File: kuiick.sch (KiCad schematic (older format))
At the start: 22 parts, among them J1 10118193-0001LF, J2 I2C_STANDARDQWIIC, J3 Conn_01x07, J4 Conn_01x07, SW1 SW_SPST, SW2 SW_SPST, U1 MK32L2B_QFN32, U2 W25Q32JVSS

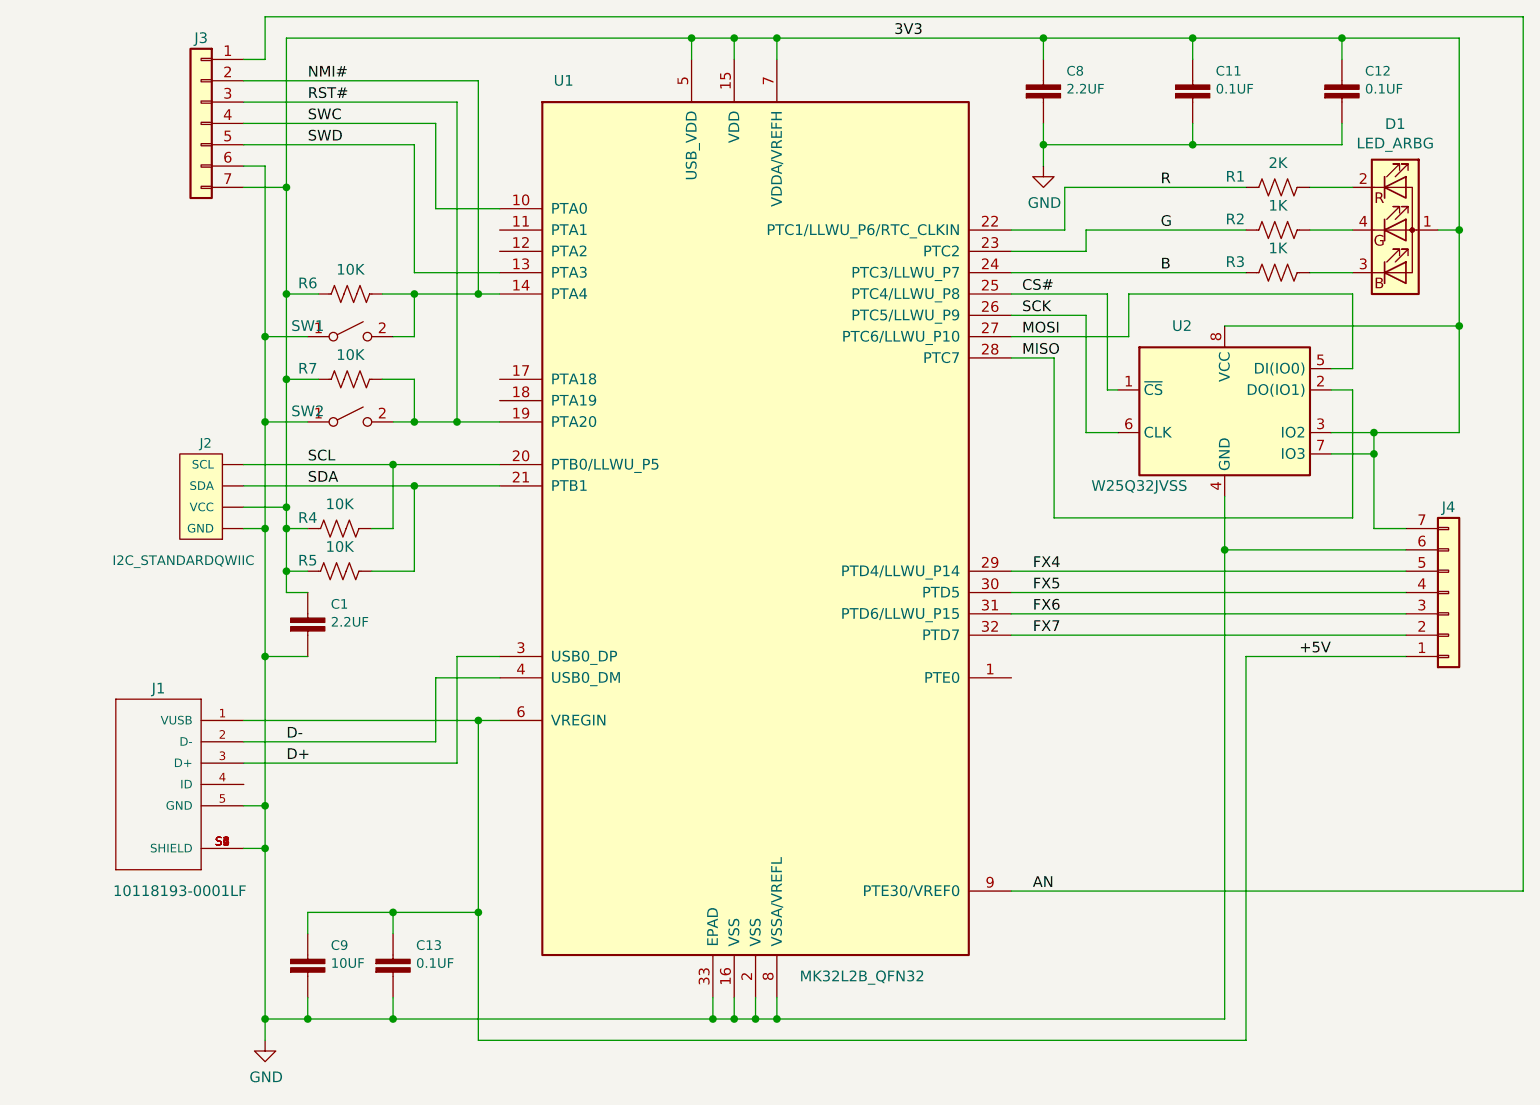
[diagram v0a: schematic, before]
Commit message: fully routed dip 16
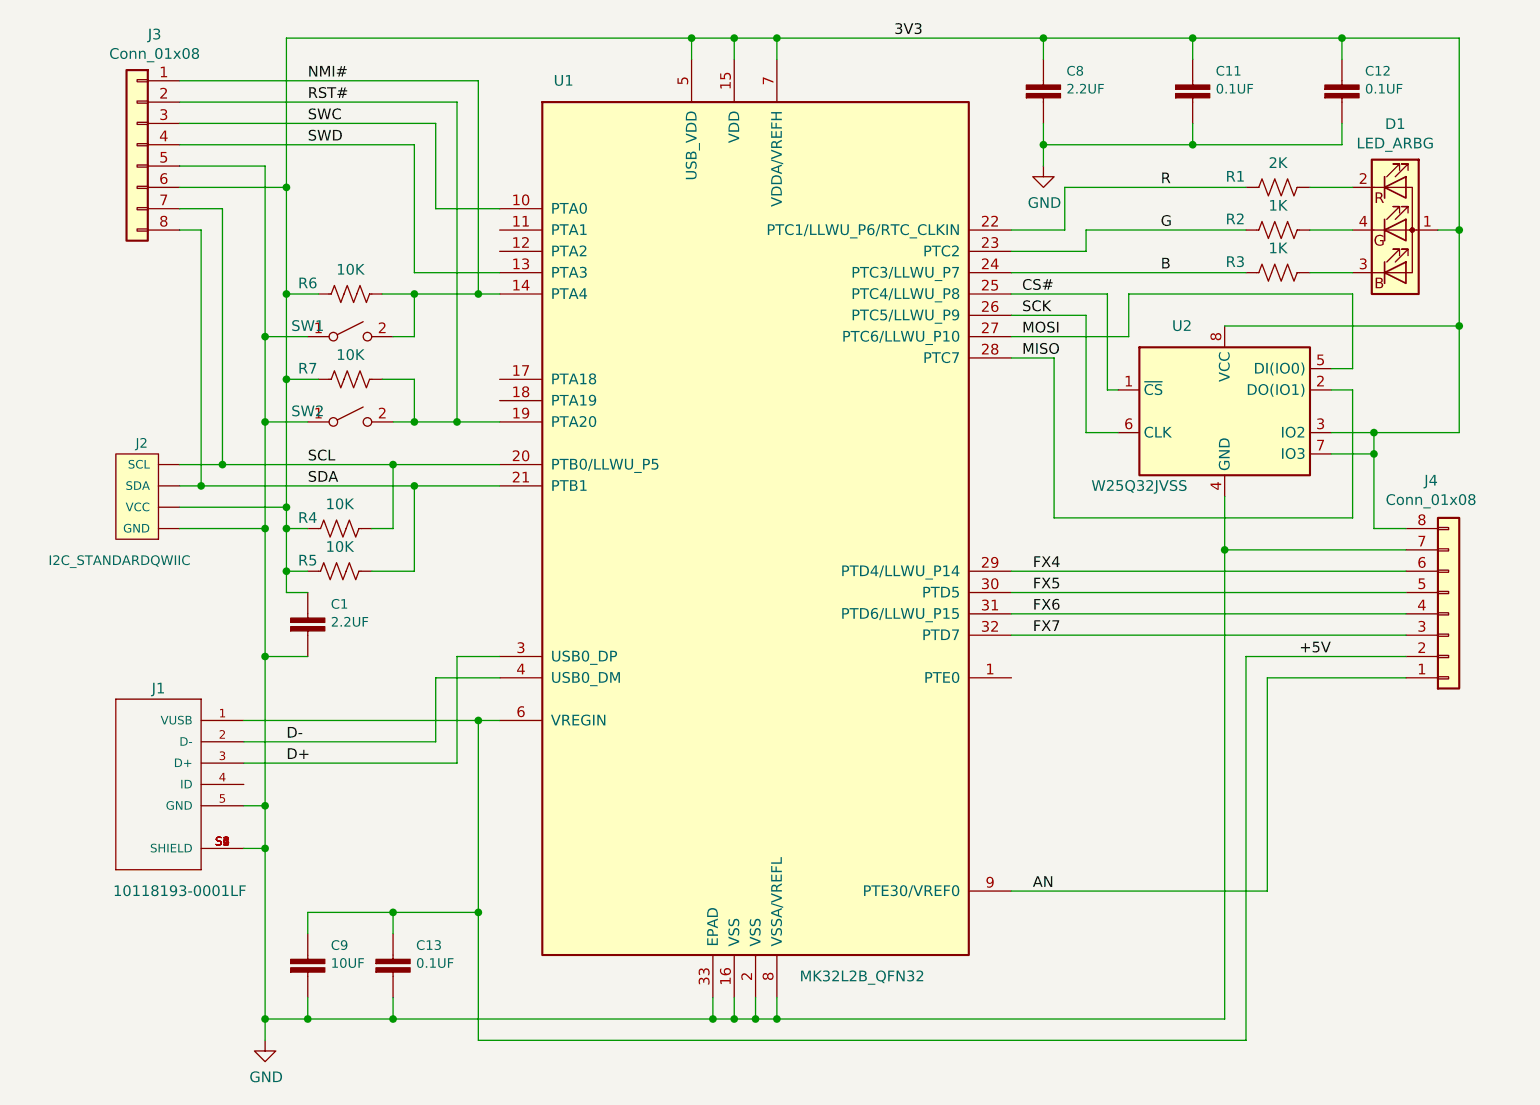
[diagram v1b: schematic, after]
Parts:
- removed J3, J4: Conn_01x07, footprint:PinHeader_1x07_P100mil_Vertical, symbol Connector_Generic:Conn_01x07
- added J3, J4: Conn_01x08, footprint:PinHeader_1x08_P100mil_Vertical, symbol Connector_Generic:Conn_01x08
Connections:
- net +5V: now also J4.2 (Pin_2)
- net 3V3: now also J3.6 (Pin_6), J4.8 (Pin_8)
- net AN: now also J4.1 (Pin_1)
- net FX4: now also J4.6 (Pin_6)
- net FX5: now also J4.5 (Pin_5)
- net FX6: now also J4.4 (Pin_4)
- net FX7: now also J4.3 (Pin_3)
- net GND: now also J3.5 (Pin_5), J4.7 (Pin_7)
- net NMI#: now also J3.1 (Pin_1)
- net RST#: now also J3.2 (Pin_2)
- net SCL: now also J3.7 (Pin_7)
- net SDA: now also J3.8 (Pin_8)
- net SWC: now also J3.3 (Pin_3)
- net SWD: now also J3.4 (Pin_4)
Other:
- moved on the sheet: J2
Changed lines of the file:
@@
-$EndComp
-$Comp
-L SparkFun-Connectors:I2C_STANDARDQWIIC J2
-U 1 1 5D51D6AB
-P 3600 3700
-F 0 "J2" H 3550 4100 45  0000 R CNN
-F 1 "I2C_STANDARDQWIIC" H 3750 3550 45  0000 R CNN
-F 2 "Connectors:1X04_1MM_RA" H 3600 4200 20  0001 C CNN
-F 3 "" H 3600 3700 50  0001 C CNN
-F 4 "CONN-13729" H 3372 3766 60  0001 R CNN "Field4"
-	1    3600 3700
-	1    0    0    -1
 $EndComp
 $Comp
@@
 $EndComp
 Wire Wire Line
-	3800 3200 3800 3700
-Wire Wire Line
 	3700 4600 4800 4600
 Connection ~ 4800 4600
@@
 Wire Wire Line
 	4700 4300 4900 4300
-$Comp
-L Connector_Generic:Conn_01x07 J3
-U 1 1 5E6EFD37
-P 3500 1800
-F 0 "J3" H 3500 2200 50  0000 C CNN
-F 1 "Conn_01x07" H 3418 2226 50  0001 C CNN
-F 2 "footprint:PinHeader_1x07_P100mil_Vertical" H 3500 1800 50  0001 C CNN
-F 3 "~" H 3500 1800 50  0001 C CNN
-	1    3500 1800
-	-1   0    0    -1
-$EndComp
-$Comp
-L Connector_Generic:Conn_01x07 J4
-U 1 1 5E6F22EF
-P 9350 4000
-F 0 "J4" H 9350 3600 50  0000 C CNN
-F 1 "Conn_01x07" H 9268 3566 50  0001 C CNN
-F 2 "footprint:PinHeader_1x07_P100mil_Vertical" H 9350 4000 50  0001 C CNN
-F 3 "~" H 9350 4000 50  0001 C CNN
-	1    9350 4000
-	1    0    0    1
-$EndComp
 Wire Wire Line
 	7300 3900 9150 3900
@@
 Wire Wire Line
 	9000 3250 9400 3250
-Wire Wire Line
-	3700 3700 3800 3700
-Connection ~ 3800 3700
 Connection ~ 3800 2800
 Wire Wire Line
 	3900 1400 3900 2100
 Wire Wire Line
-	3700 2100 3900 2100
-Wire Wire Line
-	3700 2000 3800 2000
+	3400 2100 3900 2100
+Wire Wire Line
+	3400 2000 3800 2000
 Wire Wire Line
 	3800 2000 3800 2800
@@
 	4500 2500 4900 2500
 Wire Wire Line
-	4700 1700 3700 1700
+	4700 1700 3400 1700
 Wire Wire Line
 	4800 2600 4800 1600
 Wire Wire Line
-	4800 1600 3700 1600
+	4800 1600 3400 1600
 Connection ~ 4800 2600
 Wire Wire Line
-	3700 1500 3800 1500
-Wire Wire Line
-	3800 1300 9700 1300
-Wire Wire Line
-	9700 1300 9700 5400
-Wire Wire Line
-	3800 1300 3800 1500
-Wire Wire Line
-	7300 5400 9700 5400
+	7300 5400 8500 5400
 Wire Wire Line
 	7300 2400 7650 2400
@@
 	0    1    1    0
 $EndComp
-Wire Wire Line
-	3800 3700 3800 4300
-Wire Wire Line
-	3700 3400 4400 3400
-Wire Wire Line
-	4900 3500 4500 3500
-Wire Wire Line
-	3700 3600 3900 3600
 Connection ~ 3900 2100
 Wire Wire Line
-	3900 3600 3900 3700
-Wire Wire Line
 	3900 3700 4000 3700
-Connection ~ 3900 3600
 Wire Wire Line
 	3900 3700 3900 3900
@@
 	4300 3700 4400 3700
 Wire Wire Line
-	4400 3700 4400 3400
-Connection ~ 4400 3400
-Wire Wire Line
-	4400 3400 4900 3400
-Wire Wire Line
 	4300 3900 4500 3900
-Wire Wire Line
-	4500 3900 4500 3500
-Connection ~ 4500 3500
-Wire Wire Line
-	4500 3500 3700 3500
 Wire Wire Line
 	3900 2100 3900 2600
@@
 Connection ~ 3900 3000
 Wire Wire Line
-	3900 3000 3900 3600
-Wire Wire Line
 	4350 3000 4500 3000
 Wire Wire Line
@@
 Text Label 4000 1800 0    50   ~ 0
 SWC
-Text Label 4000 3400 0    50   ~ 0
-SCL
-Text Label 4000 3500 0    50   ~ 0
-SDA
 Text Label 8000 2100 0    50   ~ 0
 R
@@
 D+
 Wire Wire Line
-	4600 1800 3700 1800
+	4600 1800 3400 1800
 Wire Wire Line
 	4600 1800 4600 2200
 Wire Wire Line
-	3700 1900 4500 1900
+	3400 1900 4500 1900
 Wire Wire Line
 	8800 3250 9000 3250
@@
 Wire Wire Line
 	9000 3350 9000 3250
+$Comp
+L Connector_Generic:Conn_01x08 J4
+U 1 1 5E82E45B
+P 9350 4100
+F 0 "J4" H 9268 3475 50  0000 C CNN
+F 1 "Conn_01x08" H 9268 3566 50  0000 C CNN
+F 2 "footprint:PinHeader_1x08_P100mil_Vertical" H 9350 4100 50  0001 C CNN
+F 3 "~" H 9350 4100 50  0001 C CNN
+	1    9350 4100
+	1    0    0    1
+$EndComp
+$Comp
+L Connector_Generic:Conn_01x08 J3
+U 1 1 5E835A4D
+P 3200 1900
+F 0 "J3" H 3118 2417 50  0000 C CNN
+F 1 "Conn_01x08" H 3118 2326 50  0000 C CNN
+F 2 "footprint:PinHeader_1x08_P100mil_Vertical" H 3200 1900 50  0001 C CNN
+F 3 "~" H 3200 1900 50  0001 C CNN
+	1    3200 1900
+	-1   0    0    -1
+$EndComp
+Wire Wire Line
+	8500 5400 8500 4400
+Wire Wire Line
+	8500 4400 9150 4400
+Wire Wire Line
+	3400 3600 3900 3600
+Wire Wire Line
+	4400 3700 4400 3400
+Connection ~ 3900 3600
+$Comp
+L SparkFun-Connectors:I2C_STANDARDQWIIC J2
+U 1 1 5D51D6AB
+P 3300 3700
+F 0 "J2" H 3250 4100 45  0000 R CNN
+F 1 "I2C_STANDARDQWIIC" H 3450 3550 45  0000 R CNN
+F 2 "Connectors:1X04_1MM_RA" H 3300 4200 20  0001 C CNN
+F 3 "" H 3300 3700 50  0001 C CNN
+F 4 "CONN-13729" H 3072 3766 60  0001 R CNN "Field4"
+	1    3300 3700
+	1    0    0    -1
+$EndComp
+Connection ~ 3800 3700
+Text Label 4000 3400 0    50   ~ 0
+SCL
+Text Label 4000 3500 0    50   ~ 0
+SDA
+Connection ~ 4400 3400
+Wire Wire Line
+	4400 3400 4900 3400
+Wire Wire Line
+	3400 3700 3800 3700
+Wire Wire Line
+	3800 3700 3800 4300
+Wire Wire Line
+	3800 3200 3800 3700
+Connection ~ 4500 3500
+Wire Wire Line
+	3900 3000 3900 3600
+Wire Wire Line
+	3900 3600 3900 3700
+Wire Wire Line
+	4500 3900 4500 3500
+Wire Wire Line
+	4900 3500 4500 3500
+Wire Wire Line
+	3400 2200 3600 2200
+Wire Wire Line
+	3400 2300 3500 2300
+Wire Wire Line
+	3400 3500 3500 3500
+Wire Wire Line
+	3400 3400 3600 3400
+Wire Wire Line
+	3500 2300 3500 3500
+Connection ~ 3500 3500
+Wire Wire Line
+	3500 3500 4500 3500
+Wire Wire Line
+	3600 2200 3600 3400
+Connection ~ 3600 3400
+Wire Wire Line
+	3600 3400 4400 3400
 $EndSCHEMATC
